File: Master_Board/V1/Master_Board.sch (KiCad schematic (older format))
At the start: 18 parts, among them J101 649022227222, Q101 BSS806NH6327XTSA1, Q102 2N7002P,215, Q103 BSS806NH6327XTSA1, Q104 BSS806NH6327XTSA1, U101 LMV321RILT, U102 LMV321RILT, U103 LMV321RILT

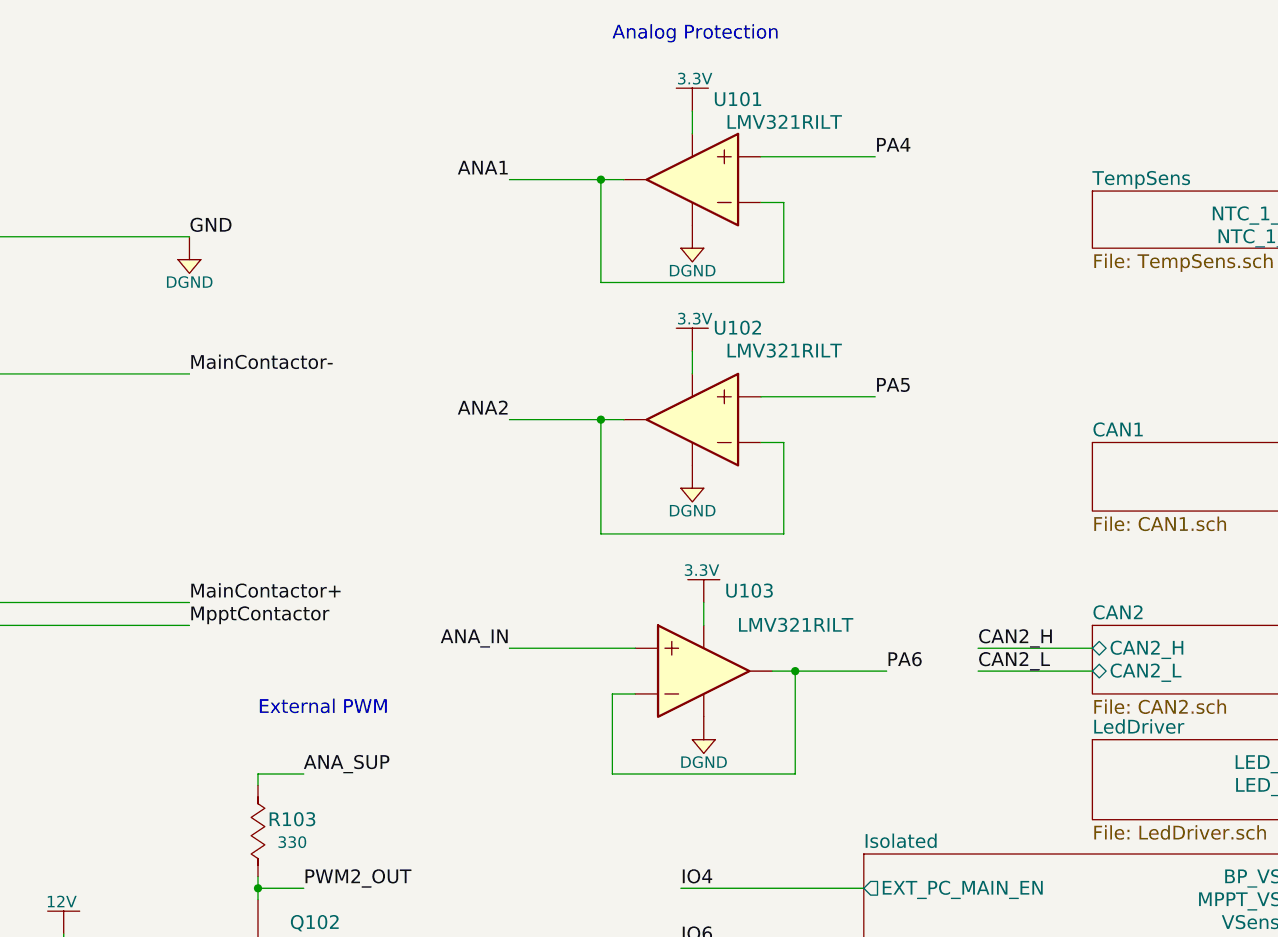
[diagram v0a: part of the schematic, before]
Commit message: Release1 MasterBoard PCB
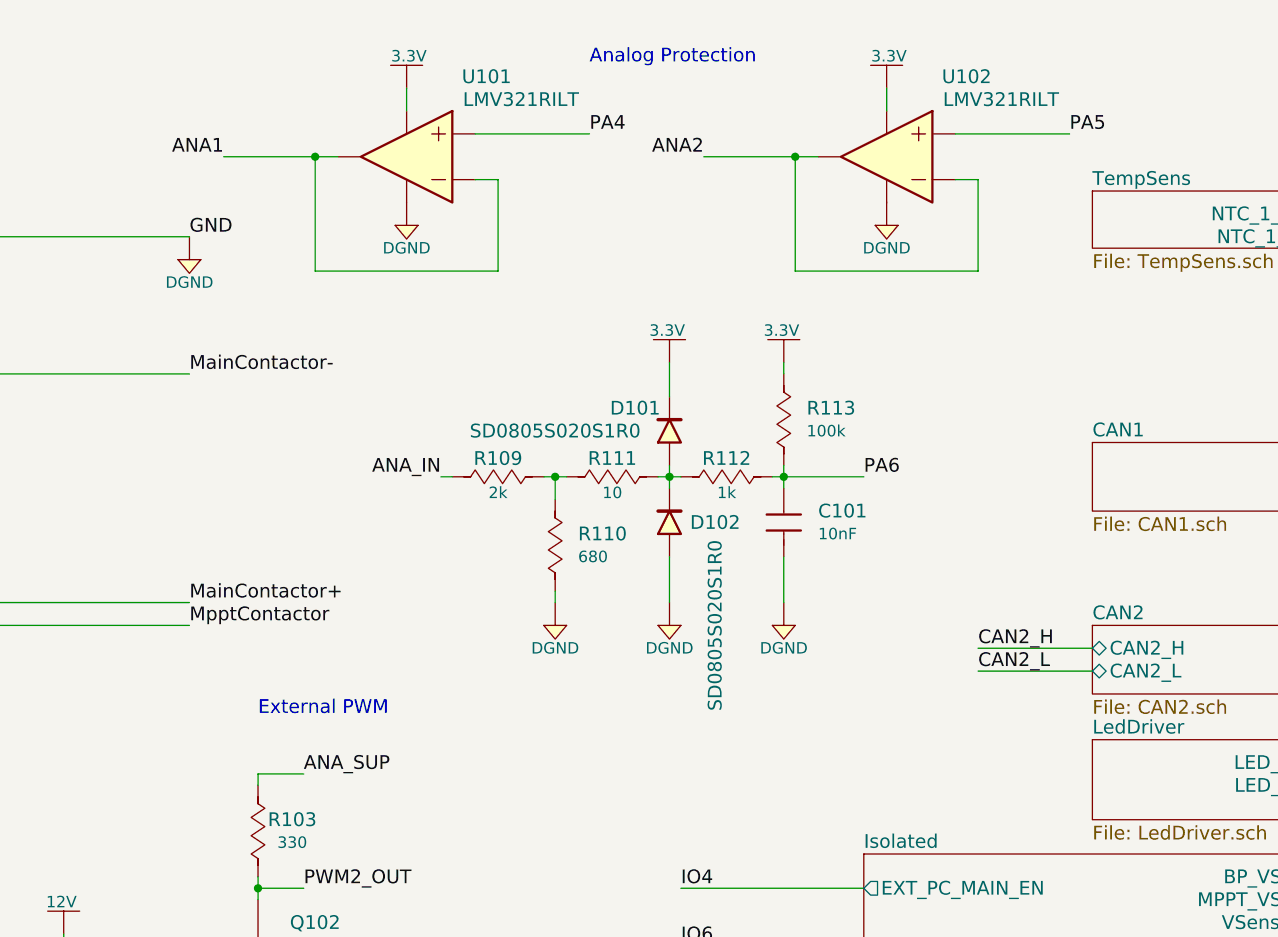
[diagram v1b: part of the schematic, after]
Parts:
- removed U103: LMV321RILT, IC:SOT-23-5, symbol LMV321RILT
- added C101: 885012207092, Capacitors:C0805, symbol 885012207092
- added D101, D102: SD0805S020S1R0, Diodes:Diode_0805, symbol SD0805S020S1R0
- added R109: RC0805JR-072KL, Resistors:R0805, symbol RC0805JR-072KL
- added R110: RC0805JR-07680RL, Resistors:R0805, symbol RC0805JR-07680RL
- added R111: RC0805JR-0710RL, Resistors:R0805, symbol RC0805JR-0710RL
- added R112: RC0805JR-071KL, Resistors:R0805, symbol RC0805JR-071KL
- added R113: RC0805JR-07100KL, Resistors:R0805, symbol RC0805JR-07100KL
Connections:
- net 3.3V: now also D101.1 (Cathode), R113.1
- net ANA_IN: now also R109.1
- net DGND: now also C101.2, D102.2 (Anode), R110.2
- net PA6: now also C101.1, R112.2, R113.2
- new net: R109.2, R110.1, R111.1
- new net: D101.2 (Anode), D102.1 (Cathode), R111.2, R112.1
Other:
- moved on the sheet: U101, U102
